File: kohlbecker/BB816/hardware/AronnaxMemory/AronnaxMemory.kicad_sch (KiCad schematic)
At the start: 37 parts, among them J1 Barrel_Jack_Switch, J2 Conn_02x40_Odd_Even, J3 Conn_02x18_Odd_Even, J4 I/O, J7 ~{IRQ7_NMI}, J8 RAM, U13 AT28C256-15PC, U2 ATF22V10, U3 ATF22V10, U4 74HC283, U5 ATF22V10, U89 74LS348

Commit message: Everything, except the plot.
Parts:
- removed C11: 100nF, Capacitor_THT:C_Disc_D3.4mm_W2.1mm_P2.50mm, symbol Device:C
- removed J7: ~{IRQ7_NMI}, symbol Connector_Generic:Conn_02x02_Odd_Even
- removed R1, R15: 1K, symbol Device:R
- removed U4: 74HC283, Package_DIP:DIP-16_W7.62mm_Socket, symbol Vega816:74HC283
- added C6, C8: 100nF, Capacitor_THT:C_Disc_D3.4mm_W2.1mm_P2.50mm, symbol Device:C
- added J9: RAM1, Connector_PinHeader_2.54mm:PinHeader_2x25_P2.54mm_Vertical, symbol Connector_Generic:Conn_02x23_Odd_Even
- added R11: 3.3k, Resistor_THT:R_Axial_DIN0207_L6.3mm_D2.5mm_P7.62mm_Horizontal, symbol Device:R_Small
- added R12: 100k, Resistor_THT:R_Axial_DIN0207_L6.3mm_D2.5mm_P7.62mm_Horizontal, symbol Device:R_Small
- added U2: 74HC74, Package_DIP:DIP-14_W7.62mm, symbol 74xx:74LS74
- added U3: 74AHC125, Package_DIP:DIP-14_W7.62mm, symbol 74xx:74LS125
- added U4: ATF22V10, Package_DIP:DIP-24_W7.62mm_Socket, symbol my:ATF22V10
- added U6: AS6C4008-55PCN, Package_DIP:DIP-32_W15.24mm_Socket, symbol Memory_RAM:AS6C4008-55PCN
- added X1: 28MHz, Oscillator:Oscillator_DIP-8, symbol Oscillator:CXO_DIP8
- J4: symbol Connector_Generic:Conn_02x18_Odd_Even -> Connector_Generic:Conn_02x16_Odd_Even
- J8: value RAM -> RAM0; footprint Connector_PinHeader_2.54mm:PinHeader_2x40_P2.54mm_Vertical -> Connector_PinHeader_2.54mm:PinHeader_2x25_P2.54mm_Vertical; symbol Connector_Generic:Conn_02x40_Odd_Even -> Connector_Generic:Conn_02x23_Odd_Even
- R14, R3, R4, R5: footprint (none) -> Resistor_THT:R_Axial_DIN0207_L6.3mm_D2.5mm_P7.62mm_Horizontal
- U7: renamed from U13; footprint Package_DIP:DIP-28_W15.24mm_Socket -> Socket:DIP_Socket-28_W11.9_W12.7_W15.24_W17.78_W18.5_3M_228-1277-00-0602J
- renumbered C12 to C21, C13 to C22, U2 to U10, U89 to U5, U3 to U8, U5 to U9
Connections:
- net ~{STRETCH} is gone; now on net ~{CLK_EN}: U9.20 (O)
- net A0: now also J8.35 (Pin_35), U8.11 (I), J9.35 (Pin_35), U6.12 (A0); no longer J8.63 (Pin_63), U8.9 (I)
- net A1: now also U8.10 (I), J9.34 (Pin_34), U4.2 (I); no longer U8.8 (I)
- net A10: now also J8.24 (Pin_24), U8.1 (CLK), J9.24 (Pin_24), U6.23 (A10); no longer J8.43 (Pin_43)
- net A11: now also J8.23 (Pin_23), J9.23 (Pin_23), U6.25 (A11); no longer J8.41 (Pin_41)
- net A12: now also J8.22 (Pin_22), J9.22 (Pin_22), U6.4 (A12); no longer J8.39 (Pin_39)
- net A13: now also J8.19 (Pin_19), J9.19 (Pin_19), U6.28 (A13); no longer J8.37 (Pin_37)
- net A14: now also J8.18 (Pin_18), J9.18 (Pin_18), U6.3 (A14); no longer J8.35 (Pin_35)
- net A15: now also J8.17 (Pin_17), J9.17 (Pin_17), U6.31 (A15); no longer J8.33 (Pin_33)
- net A16: now also J8.16 (Pin_16), J9.16 (Pin_16), U6.2 (A16); no longer J8.31 (Pin_31)
- net A17: now also J8.15 (Pin_15), J9.15 (Pin_15), U6.30 (A17); no longer J8.29 (Pin_29)
- net A18: now also J8.13 (Pin_13), J9.13 (Pin_13), U6.1 (A18); no longer J8.27 (Pin_27)
- net A19: now also J8.12 (Pin_12), J9.12 (Pin_12); no longer J8.25 (Pin_25)
- net A2: now also U8.9 (I), J9.33 (Pin_33), U4.3 (I); no longer U8.7 (I)
- net A20: now also J8.11 (Pin_11), J9.11 (Pin_11); no longer J8.23 (Pin_23)
- net A3: now also U8.8 (I), J9.32 (Pin_32), U4.4 (I); no longer U8.6 (I)
- net A4: now also U8.7 (I), J9.31 (Pin_31), U4.5 (I); no longer U8.5 (I)
- net A5: now also J8.29 (Pin_29), U8.6 (I), J9.29 (Pin_29), U6.7 (A5); no longer J8.53 (Pin_53), U8.4 (I)
- net A6: now also J8.28 (Pin_28), U8.5 (I), J9.28 (Pin_28), U6.6 (A6); no longer J8.51 (Pin_51), U8.3 (I)
- net A7: now also J8.27 (Pin_27), U8.4 (I), J9.27 (Pin_27), U6.5 (A7); no longer J8.49 (Pin_49), U8.2 (I)
- net A8: now also J8.26 (Pin_26), U8.3 (I), J9.26 (Pin_26), U6.27 (A8); no longer J8.47 (Pin_47)
- net A9: now also J8.25 (Pin_25), U8.2 (I), J9.25 (Pin_25), U6.26 (A9); no longer J8.45 (Pin_45)
- net AA1: now also J8.34 (Pin_34), U4.17 (O), U6.11 (A1); no longer J8.61 (Pin_61)
- net AA2: now also J8.33 (Pin_33), U4.18 (O), U6.10 (A2); no longer J8.59 (Pin_59)
- net AA3: now also J8.32 (Pin_32), U4.19 (O), U6.9 (A3); no longer J8.57 (Pin_57)
- net AA4: now also J8.31 (Pin_31), U4.20 (O), U6.8 (A4); no longer J8.55 (Pin_55)
- net CLK_SRC: now also R12.1, U3.8
- net D0: now also J8.45 (Pin_45), J9.45 (Pin_45), U6.13 (DQ0); no longer J8.79 (Pin_79)
- net D1: now also J8.44 (Pin_44), J9.44 (Pin_44), U6.14 (DQ1); no longer J8.77 (Pin_77)
- net D2: now also J8.43 (Pin_43), J9.43 (Pin_43), U6.15 (DQ2); no longer J8.75 (Pin_75)
- net D3: now also J8.42 (Pin_42), J9.42 (Pin_42), U6.17 (DQ3); no longer J8.73 (Pin_73)
- net D4: now also J8.41 (Pin_41), J9.41 (Pin_41), U6.18 (DQ4); no longer J8.71 (Pin_71)
- net D5: now also J8.40 (Pin_40), J9.40 (Pin_40), U6.19 (DQ5); no longer J8.69 (Pin_69)
- net D6: now also J8.39 (Pin_39), J9.39 (Pin_39), U6.20 (DQ6); no longer J8.67 (Pin_67)
- net D7: now also J8.38 (Pin_38), J9.38 (Pin_38), U6.21 (DQ7); no longer J8.65 (Pin_65)
- net E: now also R11.1, U3.10, U4.6 (I)
- net GND: now also J8.14 (Pin_14), J8.2 (Pin_2), J8.21 (Pin_21), J8.30 (Pin_30), J8.37 (Pin_37), J8.46 (Pin_46), J8.7 (Pin_7), U5.5 (EI), U8.12 (GND), C6.2, C8.2, J9.14 (Pin_14), J9.2 (Pin_2), J9.21 (Pin_21), J9.30 (Pin_30), J9.37 (Pin_37), J9.46 (Pin_46), J9.7 (Pin_7), R11.2, R12.2, U2.7 (GND), U3.7 (GND), U4.12 (GND), U6.16 (VSS), X1.4 (GND); no longer J4.10 (Pin_10), J4.14 (Pin_14), J4.18 (Pin_18), J4.2 (Pin_2), J4.22 (Pin_22), J4.26 (Pin_26), J4.30 (Pin_30), J4.34 (Pin_34), J4.36 (Pin_36), J4.6 (Pin_6)
- net VCC: now also J4.10 (Pin_10), J4.14 (Pin_14), J4.18 (Pin_18), J4.2 (Pin_2), J4.22 (Pin_22), J4.26 (Pin_26), J4.30 (Pin_30), J4.6 (Pin_6), J8.1 (Pin_1), J8.20 (Pin_20), J8.36 (Pin_36), J8.4 (Pin_4), RN1.1 (common), U8.24 (VCC), C6.1, C8.1, J9.1 (Pin_1), J9.20 (Pin_20), J9.36 (Pin_36), J9.4 (Pin_4), U2.10 (~{S}), U2.13 (~{R}), U2.14 (VCC), U3.14 (VCC), U4.24 (VCC), U6.32 (VCC), X1.8 (Vcc); no longer D3.1 (K), J4.1 (Pin_1), J4.35 (Pin_35)
- net ~{IO_0}: now also J4.1 (Pin_1); no longer J4.33 (Pin_33)
- net ~{IO_1}: now also J4.5 (Pin_5); no longer J4.29 (Pin_29)
- net ~{IO_2}: now also J4.9 (Pin_9); no longer J4.25 (Pin_25)
- net ~{IO_3}: now also J4.13 (Pin_13); no longer J4.21 (Pin_21)
- net ~{IO_5}: now also J4.21 (Pin_21); no longer J4.13 (Pin_13)
- net ~{IO_6}: now also J4.25 (Pin_25); no longer J4.9 (Pin_9)
- net ~{IO_7}: now also J4.29 (Pin_29); no longer J4.5 (Pin_5)
- net ~{IRQ0}: now also J4.3 (Pin_3), RN1.9 (R8), U5.1 (4); no longer J4.31 (Pin_31), RN1.2 (R1), U5.4 (7)
- net ~{IRQ1}: now also J4.7 (Pin_7), RN1.8 (R7), U5.2 (5); no longer J4.27 (Pin_27), RN1.3 (R2), U5.3 (6)
- net ~{IRQ2}: now also J4.11 (Pin_11), RN1.7 (R6), U5.3 (6); no longer J4.23 (Pin_23), RN1.4 (R3), U5.2 (5)
- net ~{IRQ3}: now also J4.15 (Pin_15), RN1.6 (R5), U5.4 (7); no longer J4.19 (Pin_19), RN1.5 (R4), U5.1 (4)
- net ~{IRQ4}: now also J4.19 (Pin_19), RN1.5 (R4); no longer J4.15 (Pin_15), RN1.6 (R5)
- net ~{IRQ5}: now also J4.23 (Pin_23), RN1.4 (R3); no longer J4.11 (Pin_11), RN1.7 (R6)
- net ~{IRQ6}: now also J4.27 (Pin_27), RN1.3 (R2); no longer J4.7 (Pin_7), RN1.8 (R7)
- net ~{IRQ7}: now also J4.31 (Pin_31), RN1.2 (R1), U5.10 (0); no longer J4.3 (Pin_3), RN1.9 (R8)
- net ~{IRQ}: now also U4.16 (O)
- net ~{I/O}: now also U8.13 (I); no longer U8.10 (I)
- net ~{NMI}: now also U4.21 (O); no longer D2.2 (A)
- net ~{RAM_OE}: now also J8.9 (Pin_9), J9.9 (Pin_9); no longer J8.5 (Pin_5)
- net ~{VP_REWRITE}: now also U5.15 (E0); no longer U5.5 (EI), U8.14 (O)
- net ~{VP}: now also U4.10 (I); no longer U8.11 (I)
- net ~{WR}: now also J8.10 (Pin_10), J9.10 (Pin_10); no longer J8.3 (Pin_3)
- net at R14.2, U5.14 (GS): now also D3.1 (K)
- net Y1 renamed ADDEND_AA1
- net ADDEND_AA1: now also U4.7 (I)
- net Y2 renamed ADDEND_AA2
- net ADDEND_AA2: now also U4.8 (I)
- net Y3 renamed ADDEND_AA3
- net ADDEND_AA3: now also U4.9 (I)
- net ~{MEG01} renamed ~{MEG0}
- net ~{MEG0}: now also J8.3 (Pin_3); no longer J8.21 (Pin_21)
- net ~{MEG23} renamed ~{MEG2}
- net ~{MEG2}: now also J8.5 (Pin_5); no longer J8.19 (Pin_19)
- net ~{MEG45} renamed ~{MEG4}
- net ~{MEG4}: now also J8.6 (Pin_6); no longer J8.17 (Pin_17)
- net ~{MEG67} renamed ~{MEG6}
- net ~{MEG6}: now also J8.8 (Pin_8); no longer J8.15 (Pin_15)
- net ~{MEG89} renamed ~{MEG8}
- net ~{MEG8}: now also J9.5 (Pin_5); no longer J8.13 (Pin_13)
- net ~{MEGAB} renamed ~{MEGA}
- net ~{MEGA}: now also J9.3 (Pin_3); no longer J8.11 (Pin_11)
- net ~{MEGCD} renamed ~{MEGC}
- net ~{MEGC}: now also J9.6 (Pin_6); no longer J8.9 (Pin_9)
- net ~{MEGEF} renamed ~{MEGE}
- net ~{MEGE}: now also J9.8 (Pin_8); no longer J8.7 (Pin_7)
- net ~{TURBO}: no longer names the net of U9.19 (O)
- new net: U2.12 (D), U2.8 (~{Q})
- new net 14MHz: U2.9 (Q), U3.9
- new net 28MHz: U2.11 (C), X1.5 (OUT)
- no-connect marks 3 -> 2
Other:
- note added: "2MB Boundaries"
- note added: "32KB ROM 0x008000 0x00FFFF"
- note added: "512KB RAM 0x000000 0x07FFFF"
- note added: "A1-A4 Offset"
- note added: "Address Decode - IRQ Vector Pull Rewrite - Native Mode Turbo Clock - 512KB RAM - 32KB ROM"
- note added: "BB816 System Controller"
- note added: "Bank Address"
- note added: "Based on the BB816 Breakout Board by M. Adrien Kohlbecker"
- note added: "I/O Select"
- note added: "I/O+ROM Area"
- note added: "Memory 512KB RAM + 32KB ROM"
- note added: "Native Mode Only See 65816 datasheet section 2.28"
- note added: "Note: Not subject to ~{VP} Rewrite and associated delay. See 65816 datasheet 2.28"
- note added: "Note: ~{VP} Rewrite of A1-A4 applies only to low RAM bus. See 65816 datasheet 2.28"
- note added: "Power"
- note added: "Priority"
- note added: "RAM BUS 0 Low 8 MB"
- note added: "RAM BUS 1 High 8 MB"
- note added: "Turbo Clock"
- note added: "Vector Pull Rewrite"
- note added: "~{IRQ} Pullup"
- note removed: "2 MB Segment Detection"
- note removed: "32 KB ROM 0x008000-0x00FFFF"
- note removed: "I/O CS"
- note removed: "I/O and ROM Area (Bank 0)"
- note removed: "IRQ Priority"
- note removed: "POWER"
- note removed: "RAM BUS"
- note removed: "Vector Address Rewrite"
- note removed: "~{VPB}+~{IRQ} Rewrite"
- moved on the sheet: C1, C2, C21, C22, C3, C4, C5, D1, D2, D3, H1, H2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

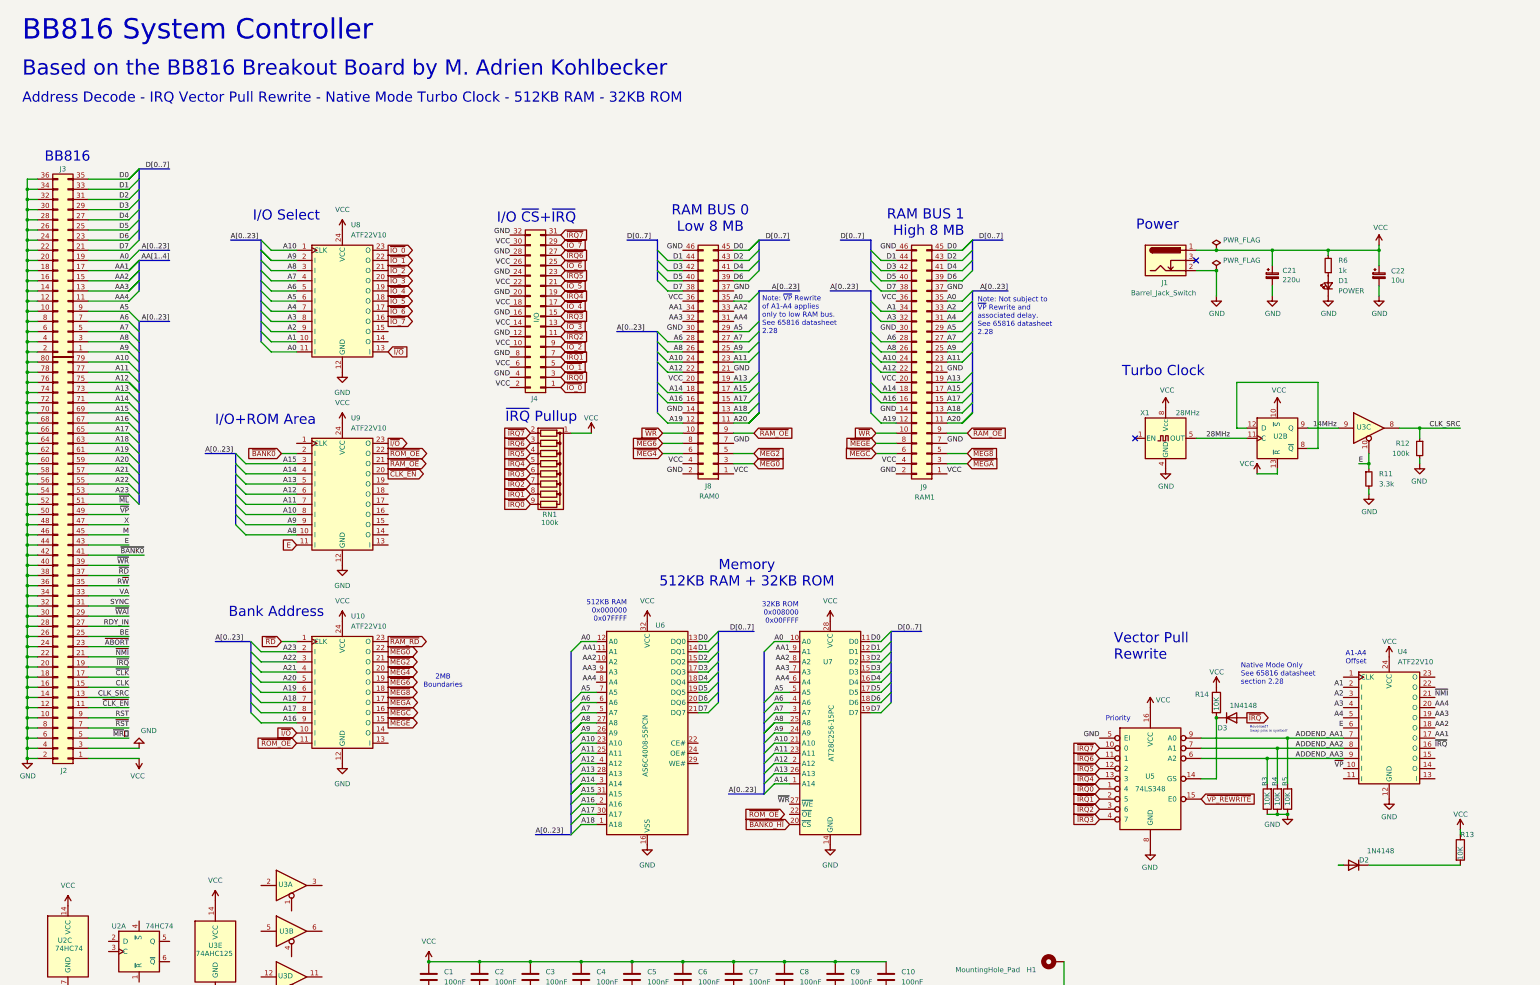
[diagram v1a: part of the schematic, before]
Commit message: Wow
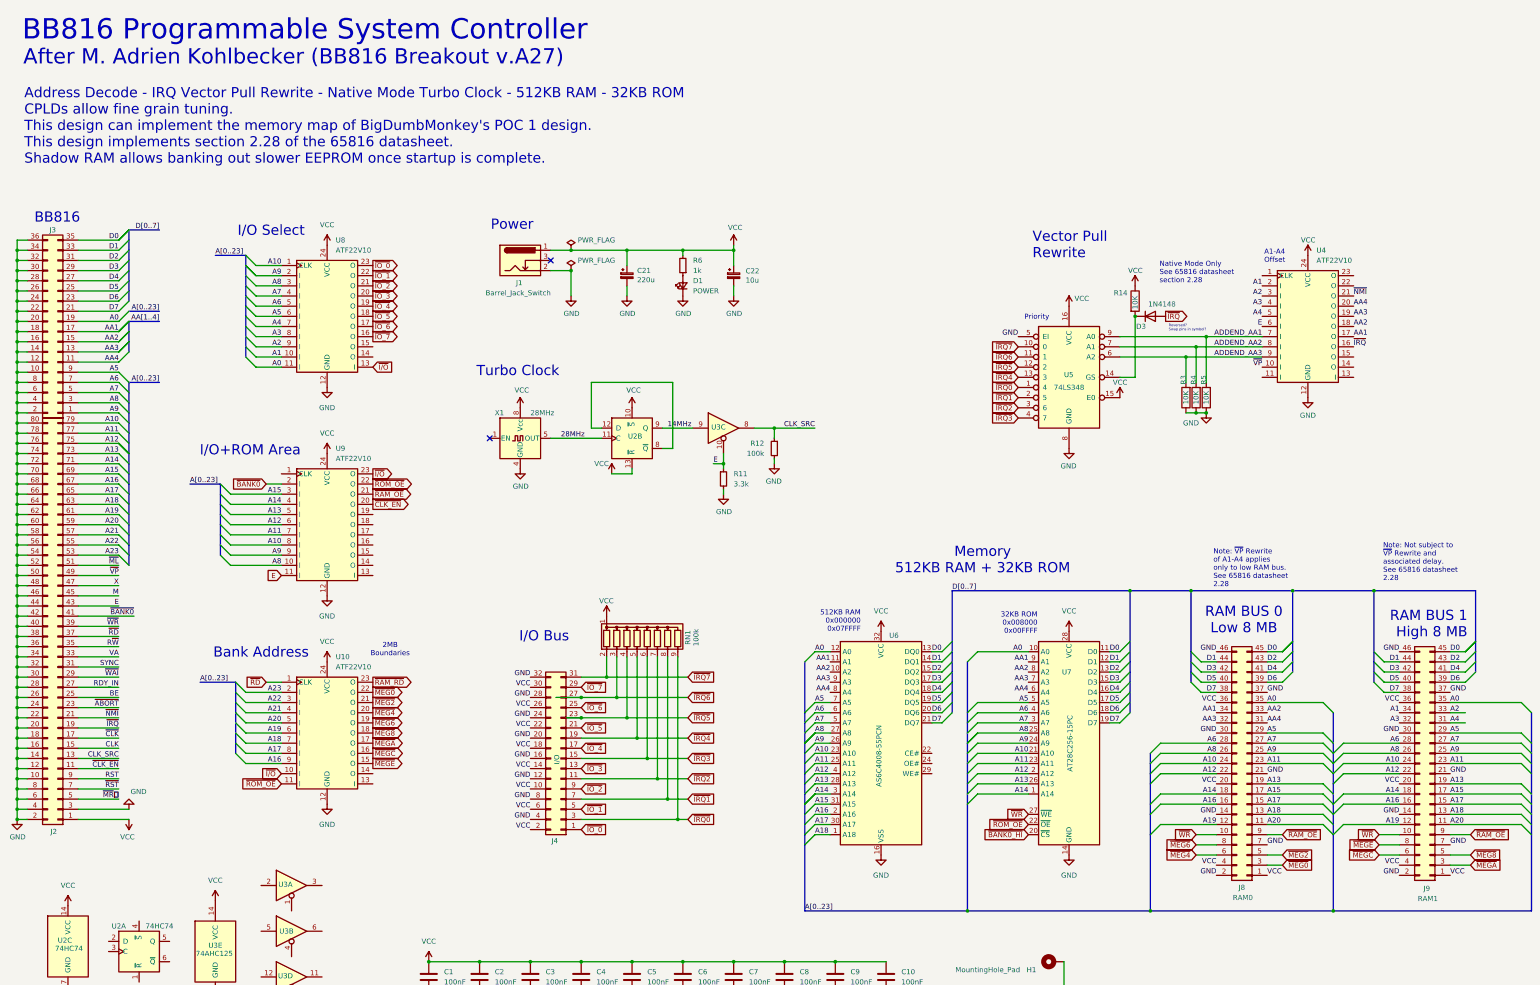
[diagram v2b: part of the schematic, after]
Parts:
- removed D2: 1N4148, Diode_THT:D_DO-35_SOD27_P7.62mm_Horizontal, symbol Diode:1N4148
- removed R13: 10K, symbol Device:R
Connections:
- net ~{VP_REWRITE} is gone; now on net VCC: U5.15 (E0)
- net ~{ROM_OE}: now also U7.22 (~{OE})
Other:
- note added: "Address Decode - IRQ Vector Pull Rewrite - Native Mode Turbo Clock - 512KB RAM - 32KB ROM CPLDs allow fine grain tuning. This design can implement the memory map of BigDumbMonkey's POC 1 design. This design implements section 2.28 of the 65816 datasheet. Shadow RAM allows banking out slower EEPROM once startup is complete."
- note added: "After M. Adrien Kohlbecker (BB816 Breakout v.A27)"
- note added: "BB816 Programmable System Controller"
- note added: "I/O Bus"
- note removed: "Address Decode - IRQ Vector Pull Rewrite - Native Mode Turbo Clock - 512KB RAM - 32KB ROM"
- note removed: "BB816 System Controller"
- note removed: "Based on the BB816 Breakout Board by M. Adrien Kohlbecker"
- note removed: "I/O ~{CS}+~{IRQ}"
- note removed: "~{IRQ} Pullup"
- moved on the sheet: C21, C22, D1, D3, J1, J2, J3, J4, J8, J9, R11, R12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
